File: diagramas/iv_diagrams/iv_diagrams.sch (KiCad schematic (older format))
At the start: 15 parts

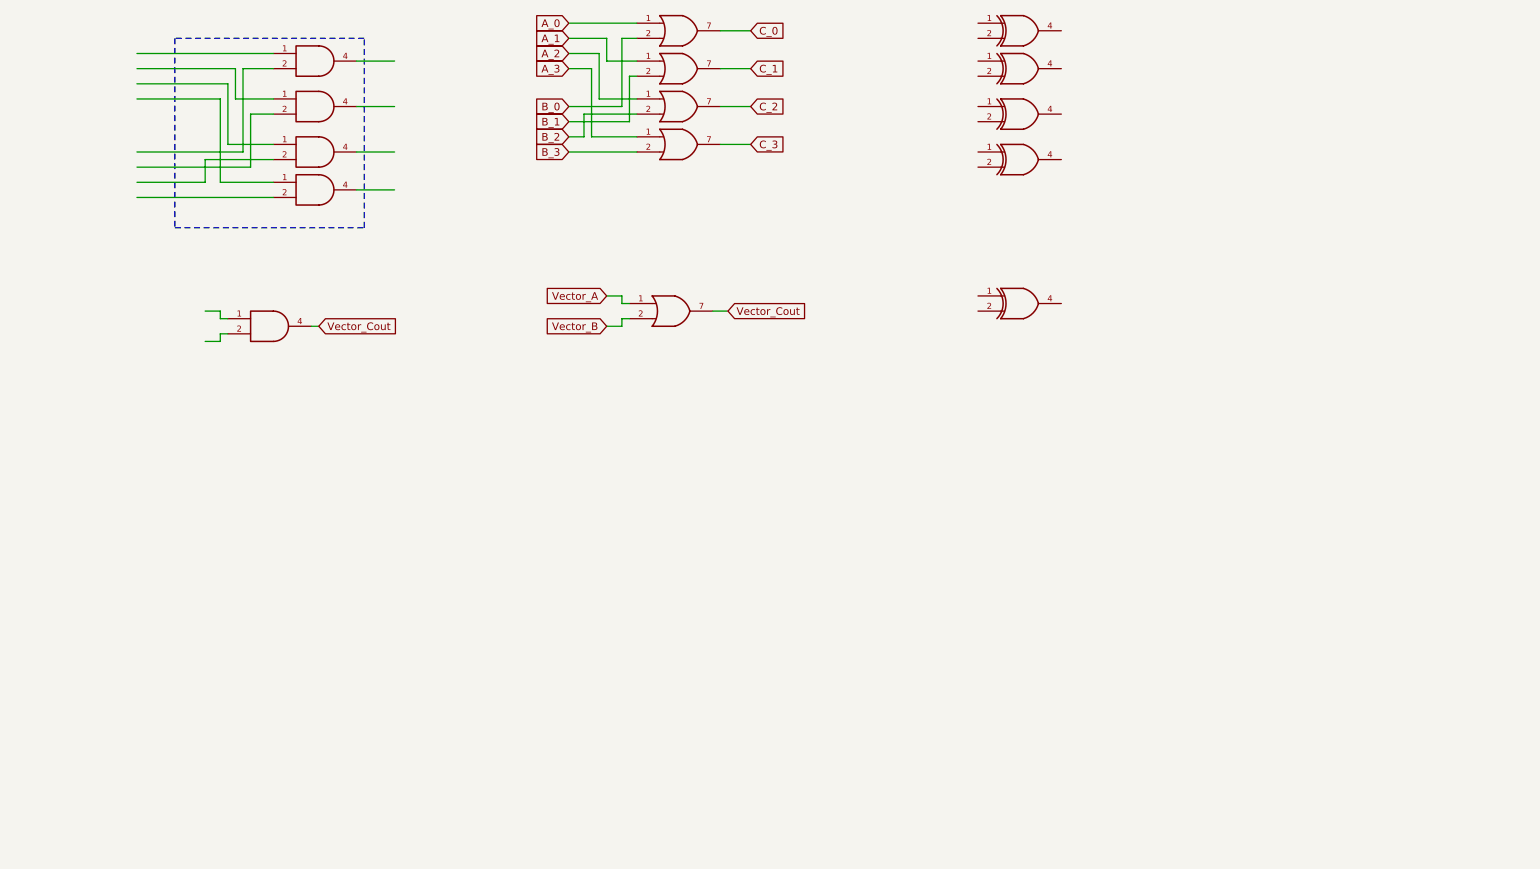
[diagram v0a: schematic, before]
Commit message: Adder with more cases
Signed-off-by: Ricardo Mena C <rgacort12@gmail.com>
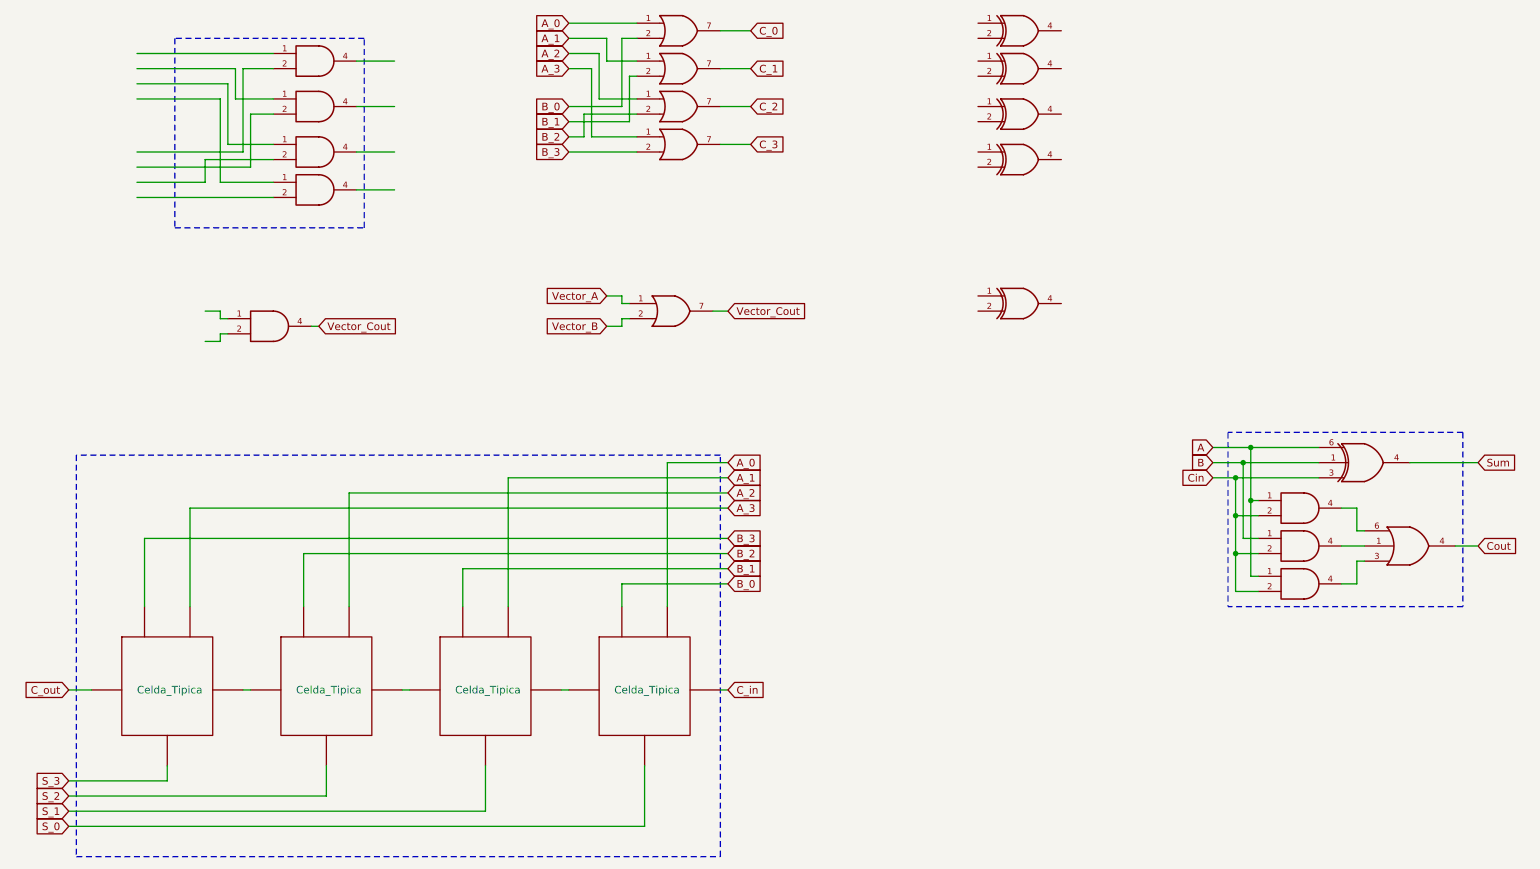
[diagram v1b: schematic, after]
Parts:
- added U? (x4): Celda_Tipica, symbol Celta_tipica:Celda_Tipica
- added U?: 74LVC1G386, symbol 74xGxx:74LVC1G386
- added U? (x3): 74AHC1G08, symbol 74xGxx:74AHC1G08
- added U?: 74LVC1G332, symbol 74xGxx:74LVC1G332
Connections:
- net labels added: A, B, C_in, C_out, Cin, Cout, S_0, S_1, S_2, S_3, Sum
- wire segments 62 -> 118
